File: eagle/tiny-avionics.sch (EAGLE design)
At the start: 61 parts, among them J1 USB-MICROB, J3 JST-PH-2-SMT-RA, U1 LP5907, U2 M25P10-AVMN6TP_TR, U5 LTC1998, U6 ATMEGA32U4-AU, X1 8MHz

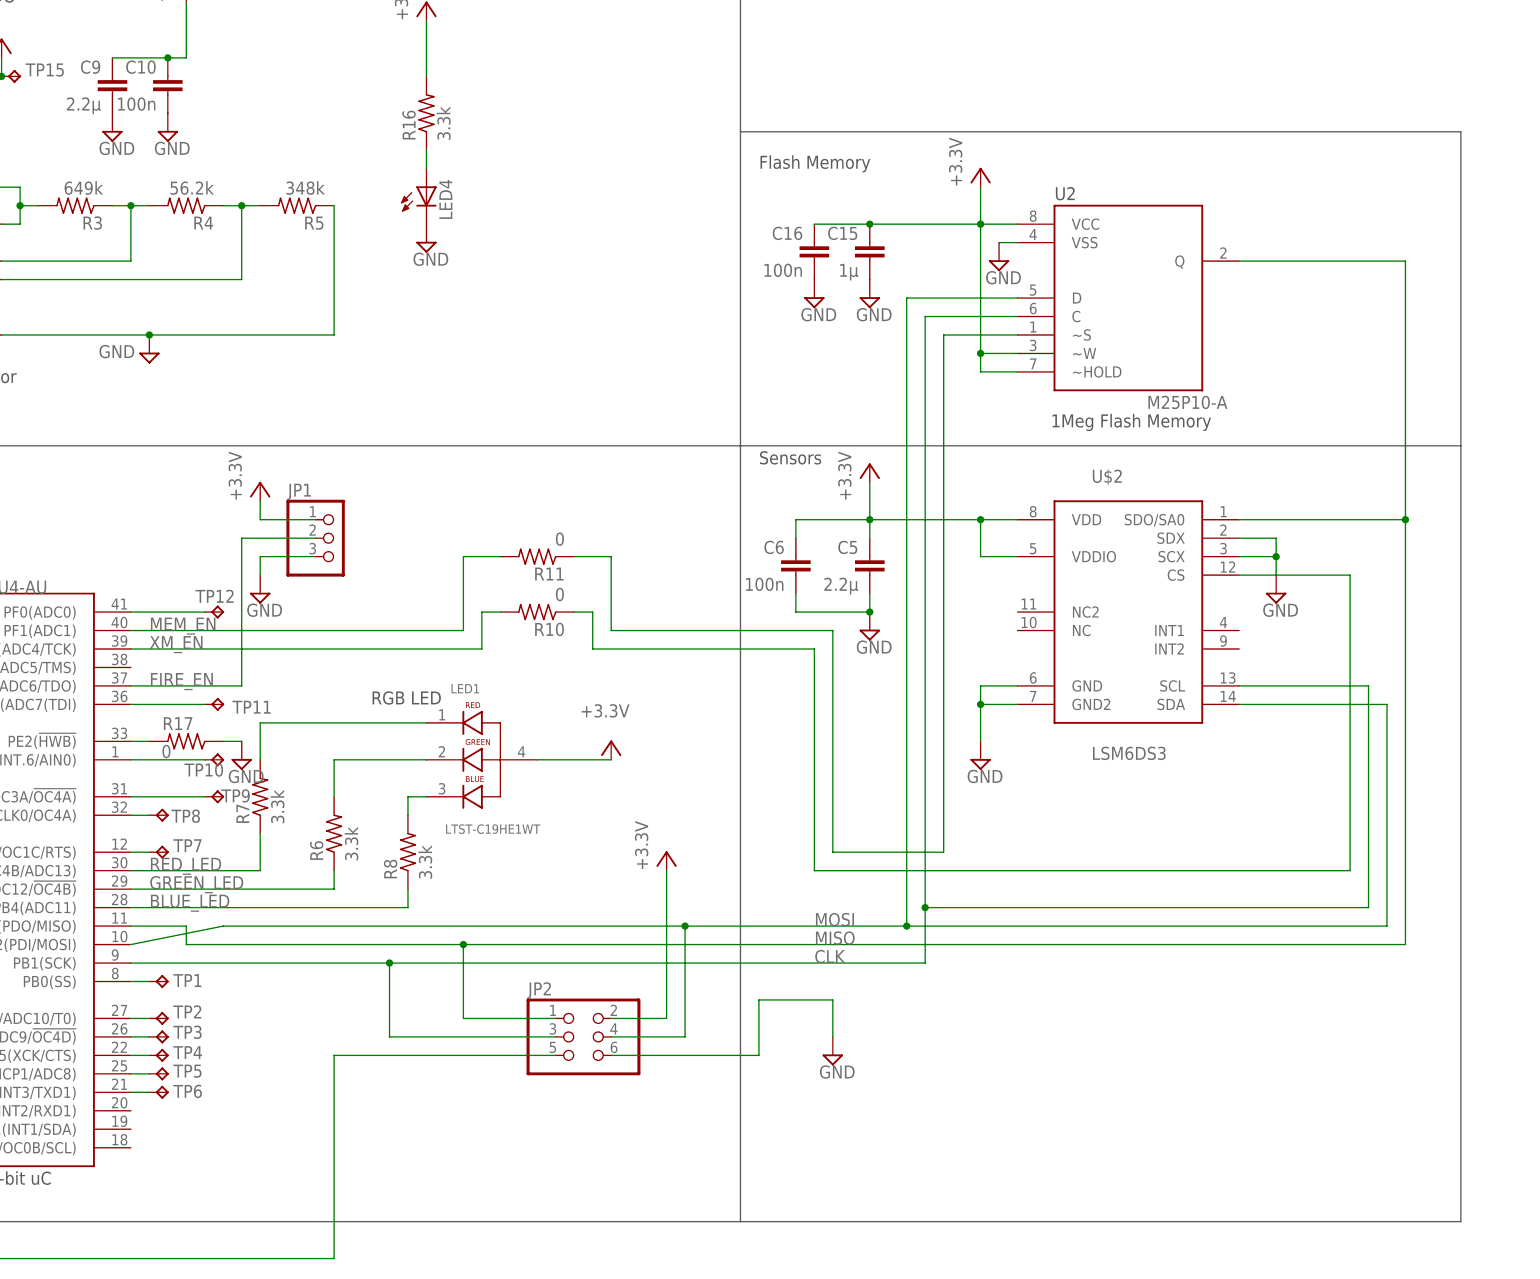
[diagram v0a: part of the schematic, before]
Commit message: Working changes to schematic and layout.
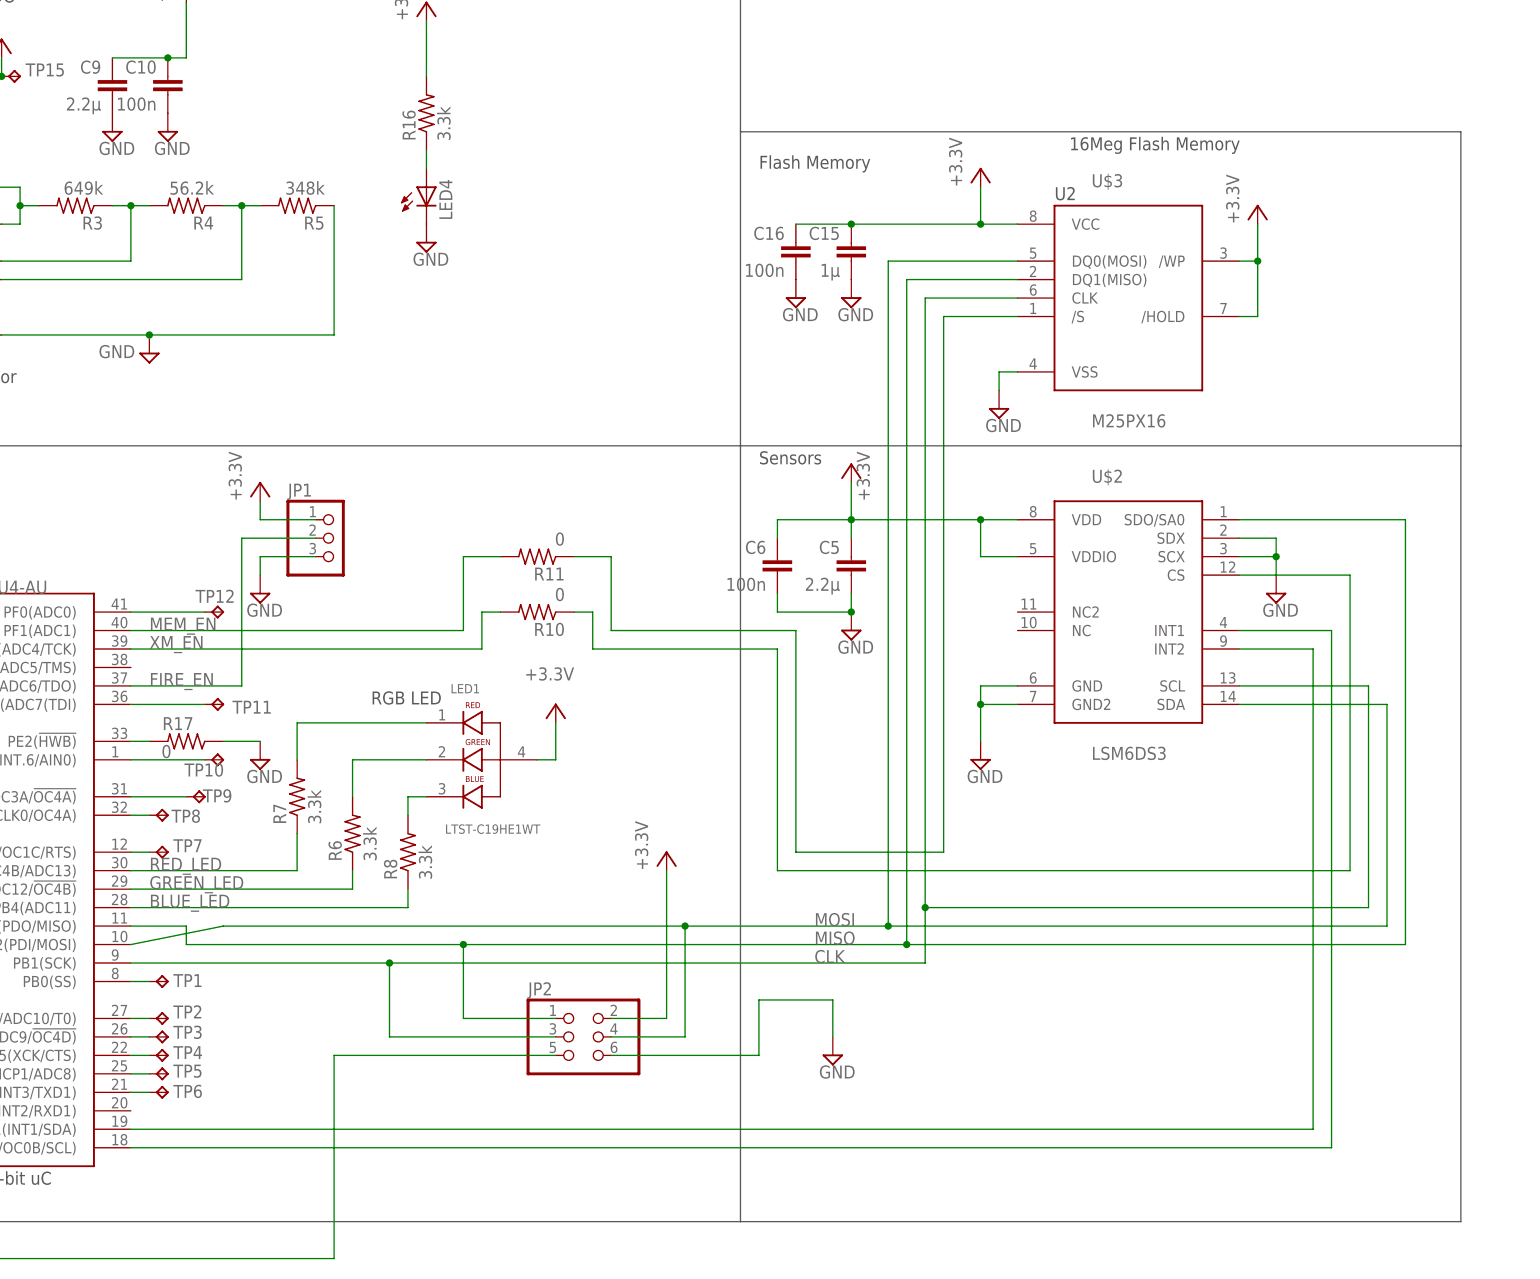
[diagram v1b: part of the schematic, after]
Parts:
- removed U2: M25P10-AVMN6TP_TR, SOIC127P600X175-8N:M25P10-AVMN6TP_TR
- added U$3: M25PX16, tinyav-lib:M25PX16
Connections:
- new net N$10: U$2.INT1, U6.PD0(INT0/OC0B/SCL)
- new net N$11: U$2.INT2, U6.PD1(INT1/SDA)
- net CLK: now also U$3.CLK; no longer U2.C
- net GND: now also U$3.VSS; no longer U2.VSS
- net MEM_EN: now also U$3./S; no longer U2.~S
- net MISO: now also U$3.DQ1(MISO); no longer U2.Q
- net MOSI: now also U$3.DQ0(MOSI); no longer U2.D
- net VCC: now also U$3./HOLD, U$3./WP, U$3.VCC; no longer U2.VCC, U2.~HOLD, U2.~W
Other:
- note added: "16Meg Flash Memory"
- note removed: "1Meg Flash Memory"
- moved on the sheet: C15, C16, C5, C6, R6, R7, TP9

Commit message: Continued layout work.
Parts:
- R1, R15: device rcl:R-US_R0805 -> rcl:R-US_R0603
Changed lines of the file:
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@@
 <grid distance="0.1" unitdist="inch" unit="inch" style="lines" multiple="1" display="no" altdistance="0.01" altunitdist="inch" altunit="inch"/>
 <layers>
-<layer number="1" name="Top" color="4" fill="1" visible="no" active="no"/>
-<layer number="16" name="Bottom" color="1" fill="1" visible="no" active="no"/>
-<layer number="17" name="Pads" color="2" fill="1" visible="no" active="no"/>
-<layer number="18" name="Vias" color="2" fill="1" visible="no" active="no"/>
-<layer number="19" name="Unrouted" color="6" fill="1" visible="no" active="no"/>
-<layer number="20" name="Dimension" color="15" fill="1" visible="no" active="no"/>
-<layer number="21" name="tPlace" color="7" fill="1" visible="no" active="no"/>
-<layer number="22" name="bPlace" color="7" fill="1" visible="no" active="no"/>
-<layer number="23" name="tOrigins" color="15" fill="1" visible="no" active="no"/>
-<layer number="24" name="bOrigins" color="15" fill="1" visible="no" active="no"/>
-<layer number="25" name="tNames" color="7" fill="1" visible="no" active="no"/>
-<layer number="26" name="bNames" color="7" fill="1" visible="no" active="no"/>
-<layer number="27" name="tValues" color="7" fill="1" visible="no" active="no"/>
-<layer number="28" name="bValues" color="7" fill="1" visible="no" active="no"/>
+<layer number="1" name="Top" color="4" fill="1" visible="yes" active="no"/>
+<layer number="16" name="Bottom" color="1" fill="1" visible="yes" active="no"/>
+<layer number="17" name="Pads" color="2" fill="1" visible="yes" active="no"/>
+<layer number="18" name="Vias" color="2" fill="1" visible="yes" active="no"/>
+<layer number="19" name="Unrouted" color="6" fill="1" visible="yes" active="no"/>
+<layer number="20" name="Dimension" color="15" fill="1" visible="yes" active="no"/>
+<layer number="21" name="tPlace" color="7" fill="1" visible="yes" active="no"/>
+<layer number="22" name="bPlace" color="7" fill="1" visible="yes" active="no"/>
+<layer number="23" name="tOrigins" color="15" fill="1" visible="yes" active="no"/>
+<layer number="24" name="bOrigins" color="15" fill="1" visible="yes" active="no"/>
+<layer number="25" name="tNames" color="7" fill="1" visible="yes" active="no"/>
+<layer number="26" name="bNames" color="7" fill="1" visible="yes" active="no"/>
+<layer number="27" name="tValues" color="7" fill="1" visible="yes" active="no"/>
+<layer number="28" name="bValues" color="7" fill="1" visible="yes" active="no"/>
 <layer number="29" name="tStop" color="7" fill="3" visible="no" active="no"/>
 <layer number="30" name="bStop" color="7" fill="6" visible="no" active="no"/>
@@
 <layer number="35" name="tGlue" color="7" fill="4" visible="no" active="no"/>
 <layer number="36" name="bGlue" color="7" fill="5" visible="no" active="no"/>
-<layer number="37" name="tTest" color="7" fill="1" visible="no" active="no"/>
-<layer number="38" name="bTest" color="7" fill="1" visible="no" active="no"/>
+<layer number="37" name="tTest" color="7" fill="1" visible="yes" active="no"/>
+<layer number="38" name="bTest" color="7" fill="1" visible="yes" active="no"/>
 <layer number="39" name="tKeepout" color="4" fill="11" visible="no" active="no"/>
 <layer number="40" name="bKeepout" color="1" fill="11" visible="no" active="no"/>
@@
 <layer number="44" name="Drills" color="7" fill="1" visible="no" active="no"/>
 <layer number="45" name="Holes" color="7" fill="1" visible="no" active="no"/>
-<layer number="46" name="Milling" color="3" fill="1" visible="no" active="no"/>
-<layer number="47" name="Measures" color="7" fill="1" visible="no" active="no"/>
-<layer number="48" name="Document" color="7" fill="1" visible="no" active="no"/>
-<layer number="49" name="Reference" color="7" fill="1" visible="no" active="no"/>
-<layer number="50" name="dxf" color="7" fill="1" visible="no" active="no"/>
-<layer number="51" name="tDocu" color="7" fill="1" visible="no" active="no"/>
-<layer number="52" name="bDocu" color="7" fill="1" visible="no" active="no"/>
-<layer number="53" name="tGND_GNDA" color="7" fill="9" visible="no" active="no"/>
-<layer number="54" name="bGND_GNDA" color="1" fill="9" visible="no" active="no"/>
-<layer number="56" name="wert" color="7" fill="1" visible="no" active="no"/>
-<layer number="57" name="tCAD" color="7" fill="1" visible="no" active="no"/>
-<layer number="59" name="tCarbon" color="7" fill="1" visible="no" active="no"/>
-<layer number="60" name="bCarbon" color="7" fill="1" visible="no" active="no"/>
+<layer number="46" name="Milling" color="3" fill="1" visible="yes" active="no"/>
+<layer number="47" name="Measures" color="7" fill="1" visible="yes" active="no"/>
+<layer number="48" name="Document" color="7" fill="1" visible="yes" active="no"/>
+<layer number="49" name="Reference" color="7" fill="1" visible="yes" active="no"/>
+<layer number="50" name="dxf" color="7" fill="1" visible="yes" active="no"/>
+<layer number="51" name="tDocu" color="7" fill="1" visible="yes" active="no"/>
+<layer number="52" name="bDocu" color="7" fill="1" visible="yes" active="no"/>
+<layer number="53" name="tGND_GNDA" color="7" fill="9" visible="yes" active="no"/>
+<layer number="54" name="bGND_GNDA" color="1" fill="9" visible="yes" active="no"/>
+<layer number="56" name="wert" color="7" fill="1" visible="yes" active="no"/>
+<layer number="57" name="tCAD" color="7" fill="1" visible="yes" active="no"/>
+<layer number="59" name="tCarbon" color="7" fill="1" visible="yes" active="no"/>
+<layer number="60" name="bCarbon" color="7" fill="1" visible="yes" active="no"/>
 <layer number="90" name="Modules" color="5" fill="1" visible="yes" active="yes"/>
 <layer number="91" name="Nets" color="2" fill="1" visible="yes" active="yes"/>
@@
 <part name="R13" library="rcl" deviceset="R-US_" device="R0603" value="22"/>
 <part name="LED2" library="adafruit" deviceset="LED" device="CHIP-LED0603"/>
-<part name="R15" library="rcl" deviceset="R-US_" device="R0805" value="3.3k"/>
+<part name="R15" library="rcl" deviceset="R-US_" device="R0603" value="3.3k"/>
 <part name="JP2" library="pinhead" deviceset="PINHD-2X3" device=""/>
 <part name="SUPPLY8" library="supply2" deviceset="GND" device=""/>
@@
 <part name="U$1" library="tinyav-lib" deviceset="BQ21040" device=""/>
 <part name="SUPPLY1" library="supply2" deviceset="GND" device=""/>
-<part name="R1" library="rcl" deviceset="R-US_" device="R0805" value="5.36k"/>
+<part name="R1" library="rcl" deviceset="R-US_" device="R0603" value="5.36k"/>
 <part name="SUPPLY3" library="supply2" deviceset="GND" device=""/>
 <part name="U$2" library="tinyav-lib" deviceset="LSM6DS3" device=""/>
